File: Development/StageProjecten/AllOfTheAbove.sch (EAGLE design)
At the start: 90 parts, among them IC1 7809DT, IC2 TL074TSSOP14, IC3 TL074TSSOP14, IC4 TL074TSSOP14, IC5 UA741D, J1 JACK, J10 JACK, J11 JACK, J12 JACK, J13 JACK, J14 JACK, J15 JACK, J16 JACK, J2 POWERSHROUDED, J3 JACK, J4 JACK, J5 JACK, J6 JACK, J7 JACK, J8 JACK, J9 JACK

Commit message: Rat added with powerjumpers
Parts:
- added C29, C30, C31, C32, C33, C34, C35, C36, C37, C38, C39: (no value), OPL:C-0603
- added D13, D14: (no value), OPL:D-D1206
- added IC6: UA741D, linear:UA741D
- added JP1, JP2, JP3: (no value), pinhead:PINHD-1X3
- added Q1: SST201, transistor-fet:SST201
- added R22, R29, R30, R31: (no value), EurorackModularParts:POTSQUAREHOLE_SMALLKNOB
- added R32, R33, R34, R35, R36, R37, R38, R39, R40: (no value), OPL:R-0603
- D11, D12: device diode:DIODE-DO-214AC -> OPL:D-D1206
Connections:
- new net +4.5V: R34.2
- new net N$36: R22.E, R22.S, R28.1
- new net N$37: C29.2, JP1.2, R33.1
- new net N$38: C30.2, IC6.+IN, R33.2
- new net N$39: IC6.V+, JP2.2
- new net N$40: IC6.V-, JP3.2
- new net N$41: JP1.1, R34.1
- new net N$42: C31.1, IC6.-IN, R31.E, R31.S, R35.2, R36.2
- new net N$43: C31.2, C34.2, IC6.OUT, R31.A
- new net N$44: C34.1, R37.1
- new net N$45: D13.-, D14.+, R30.E, R30.S, R37.2
- new net N$46: R30.A, R38.1
- new net N$47: C33.2, R36.1
- new net N$48: C32.2, R35.1
- new net N$49: C35.1, C36.1, R38.2
- new net N$50: C36.2, Q1.G, R39.2
- new net N$51: C37.1, Q1.S, R40.2
- new net N$52: C37.2, R29.A
- net -12V: now also C39.1, JP3.3
- net 12V: now also C38.2, JP2.3
- net 9V: now also JP2.1, Q1.D
- net GND: now also C30.1, C32.1, C33.1, C35.2, C38.1, C39.2, D11.+, D12.-, D13.+, D14.-, JP3.1, R29.E, R32.2, R39.1, R40.1; no longer D11.A, D12.C
- net INPUT_B: now also C29.1, R32.1
- net N$21: now also IC5.+IN; no longer IC5.-IN
- net N$22: now also IC5.-IN; no longer IC5.+IN
- net N$34: now also D11.-, D12.+, R22.A; no longer D11.C, D12.A, R28.1

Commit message: Added FF&Muff schematic (.brd not updated)
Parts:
- added C40, C41, C42, C43, C44, C45, C46, C47, C48, C49, C50, C51, C52, C53, C54, C55: (no value), OPL:C-0603
- added D15, D16, D17, D18: (no value), OPL:D-D1206
- added Q2, Q3: BCX71SMD, transistor-pnp:BCX71SMD
- added Q4, Q5, Q6, Q7: BC849SMD, transistor-npn:BC849SMD
- added R41, R44, R45, R46, R47, R48, R49, R50, R51, R52, R53, R54, R55, R56, R57, R58, R59, R60, R61, R62, R63, R64, R65, R66, R67, R68: (no value), OPL:R-0603
- added R42, R43, R69, R70, R71: (no value), EurorackModularParts:POTSQUAREHOLE_SMALLKNOB
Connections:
- new net N$53: Q3.E, R41.1, R43.A
- new net N$54: C40.2, Q2.B, R41.2
- new net N$55: Q2.C, Q3.B, R45.2
- new net N$56: C41.1, R43.S
- new net N$57: C42.2, R42.A
- new net N$58: C42.1, R44.1, R46.2
- new net N$59: Q3.C, R44.2
- new net N$60: C43.1, R47.2
- new net N$61: C43.2, C44.1, Q4.B, R48.2, R49.2
- new net N$62: Q4.E, R50.1
- new net N$63: C44.2, C45.1, Q4.C, R49.1, R51.2
- new net N$64: C45.2, R71.A
- new net N$65: C47.1, C48.1, Q5.B, R53.2, R54.2, R56.2
- new net N$66: C48.2, D15.+, D16.-
- new net N$67: Q5.E, R55.2
- new net N$68: C47.2, C49.1, D15.-, D16.+, Q5.C, R56.1, R57.2
- new net N$69: C49.2, R58.1
- new net N$70: C50.1, C51.1, Q6.B, R58.2, R59.2, R61.2
- new net N$71: Q6.E, R60.2
- new net N$72: C50.2, C52.1, D17.-, D18.+, Q6.C, R61.1, R62.2, R63.1
- new net N$73: C53.1, R70.S
- new net N$74: C55.2, R63.2, R70.E
- new net N$75: C52.2, R64.1, R70.A
- new net N$76: C51.2, D17.+, D18.-
- new net N$77: C53.2, Q7.B, R65.2, R66.1
- new net N$78: C54.1, Q7.C, R67.1
- new net N$79: Q7.E, R68.2
- new net N$80: C54.2, R69.A
- new net N$84: R52.1, R71.E
- new net N$85: C46.2, R53.1
- new net N$86: C46.1, R71.S
- net 9V: now also R45.1, R46.1, R51.1, R57.1, R62.1, R66.2, R67.2
- net GND: now also C41.2, C55.1, Q2.E, R42.E, R43.E, R48.1, R50.2, R52.2, R54.1, R55.1, R59.1, R60.1, R64.2, R65.1, R68.1, R69.E
- net INPUT_C: now also C40.1
- net INPUT_D: now also R47.1
- net OUTPUT_B: now also R29.S
- net OUTPUT_C: now also R42.S
- net OUTPUT_D: now also R69.S

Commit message: Added Modules/Guitar In
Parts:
- removed C28, C29, C30, C31, C32, C33, C34, C35, C36, C37, C38, C39, C40, C41, C42, C43, C44, C45, C46, C47, C48, C49, C50, C51, C52, C53, C54, C55: (no value), OPL:C-0603
- removed D11, D12, D13, D14, D15, D16, D17, D18: (no value), OPL:D-D1206
- removed IC6: UA741D, linear:UA741D
- removed JP1, JP2, JP3: (no value), pinhead:PINHD-1X3
- removed Q1: SST201, transistor-fet:SST201
- removed Q2, Q3: BCX71SMD, transistor-pnp:BCX71SMD
- removed Q4, Q5, Q6, Q7: BC849SMD, transistor-npn:BC849SMD
- removed R27, R28, R32, R33, R34, R35, R36, R37, R38, R39, R40, R41, R44, R45, R46, R47, R48, R49, R50, R51, R52, R53, R54, R55, R56, R57, R58, R59, R60, R61, R62, R63, R64, R65, R66, R67, R68: (no value), OPL:R-0603
- removed R29, R30, R31, R42, R43, R69, R70, R71: (no value), EurorackModularParts:POTSQUAREHOLE_SMALLKNOB
- C22: value (none) -> 10uF
- IC5: value UA741D -> TL071D; device linear:UA741D -> EurorackModularParts:TL071D
- R22: value (none) -> 1M; device EurorackModularParts:POTSQUAREHOLE_SMALLKNOB -> OPL:R-0603; DESC Tone -> (none)
- R23: value 1M -> 150K; device EurorackModularParts:POTSQUAREHOLE_SMALLKNOB -> OPL:R-0603; DESC Distortion -> (none)
- R24: value 10K -> (none); device EurorackModularParts:POTSQUAREHOLE_SMALLKNOB -> OPL:R-0603; DESC Volume -> (none)
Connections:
- removed net +4.5V: R34.2
- removed net N$37: C29.2, JP1.2, R33.1
- removed net N$39: IC6.V+, JP2.2
- removed net N$40: IC6.V-, JP3.2
- removed net N$41: JP1.1, R34.1
- removed net N$42: C31.1, IC6.-IN, R31.E, R31.S, R35.2, R36.2
- removed net N$43: C31.2, C34.2, IC6.OUT, R31.A
- removed net N$44: C34.1, R37.1
- removed net N$45: D13.-, D14.+, R30.E, R30.S, R37.2
- removed net N$46: R30.A, R38.1
- removed net N$47: C33.2, R36.1
- removed net N$48: C32.2, R35.1
- removed net N$49: C35.1, C36.1, R38.2
- removed net N$50: C36.2, Q1.G, R39.2
- removed net N$51: C37.1, Q1.S, R40.2
- removed net N$52: C37.2, R29.A
- removed net N$53: Q3.E, R41.1, R43.A
- removed net N$54: C40.2, Q2.B, R41.2
- removed net N$55: Q2.C, Q3.B, R45.2
- removed net N$56: C41.1, R43.S
- removed net N$57: C42.2, R42.A
- removed net N$58: C42.1, R44.1, R46.2
- removed net N$59: Q3.C, R44.2
- removed net N$60: C43.1, R47.2
- removed net N$61: C43.2, C44.1, Q4.B, R48.2, R49.2
- removed net N$62: Q4.E, R50.1
- removed net N$63: C44.2, C45.1, Q4.C, R49.1, R51.2
- removed net N$64: C45.2, R71.A
- removed net N$65: C47.1, C48.1, Q5.B, R53.2, R54.2, R56.2
- removed net N$66: C48.2, D15.+, D16.-
- removed net N$67: Q5.E, R55.2
- removed net N$68: C47.2, C49.1, D15.-, D16.+, Q5.C, R56.1, R57.2
- removed net N$69: C49.2, R58.1
- removed net N$70: C50.1, C51.1, Q6.B, R58.2, R59.2, R61.2
- removed net N$71: Q6.E, R60.2
- removed net N$72: C50.2, C52.1, D17.-, D18.+, Q6.C, R61.1, R62.2, R63.1
- removed net N$73: C53.1, R70.S
- removed net N$74: C55.2, R63.2, R70.E
- removed net N$75: C52.2, R64.1, R70.A
- removed net N$76: C51.2, D17.+, D18.-
- removed net N$77: C53.2, Q7.B, R65.2, R66.1
- removed net N$78: C54.1, Q7.C, R67.1
- removed net N$79: Q7.E, R68.2
- removed net N$80: C54.2, R69.A
- removed net N$84: R52.1, R71.E
- removed net N$85: C46.2, R53.1
- removed net N$86: C46.1, R71.S
- new net BIASMAINLINE: C7.1, D2.ANODE, D4.ANODE, D6.ANODE, D7.ANODE, D8.ANODE, IC1.OUT, R13.1
- new net GUITAR_IN: C22.1, R22.2
- new net GUITAR_OUT: R26.2
- new net INPUT_E: R14.2
- new net N$81: IC5.V+
- new net N$82: IC5.V-
- new net OUTPUT_E: R22.1, R23.1
- net -12V: now also C27.1, C4.1, C6.1, IC1.V-, IC3SUPPLY.V-, R12.1, R9.2, U$13.-12V; no longer C39.1, IC5.V-, JP3.3
- net 12V: now also C26.2, C3.2, C5.2, IC1.V+, IC3SUPPLY.V+, R2.A; no longer C38.2, IC5.V+, JP2.3
- net 9V: no longer JP2.1, Q1.D, R45.1, R46.1, R51.1, R57.1, R62.1, R66.2, R67.2
- net GND: now also C23.1, C25.1, C26.1, C27.2, C3.1, C4.2, C6.2, D1.CATHODE, D10.CATHODE, D3.CATHODE, D5.CATHODE, D9.CATHODE, IC1.+IN, IC3BUF1.B, IC3BUF2.B, IC3OTA2.IN_N, IC3OTA2.IN_P, R1.E, R2.E, R22.1, R23.1, R24.2, R25.1, R26.1, R4.2, R5.2, R7.1, R8.1; no longer C28.1, C30.1, C32.1, C33.1, C35.2, C38.1, C39.2, C41.2, C55.1, D11.+, D12.-, D13.+, D14.-, JP3.1, Q2.E, R29.E, R32.2, R39.1, R40.1, R42.E, R43.E, R48.1, R50.2, R52.2, R54.1, R55.1, R59.1, R60.1, R64.2, R65.1, R68.1, R69.E
- net INPUT_B: no longer C29.1, R32.1
- net INPUT_C: no longer C40.1
- net INPUT_D: no longer R47.1
- net N$1: now also R4.1
- net N$10: now also R6.1
- net N$11: now also C8.1, IC1.OUT, R15.1, R16.2, R17.2
- net N$12: now also C14.2, C8.2, IC1.-IN, R15.2
- net N$13: now also C14.1, IC3OTA1.OUT, R5.1
- net N$14: now also D3.ANODE, D4.CATHODE, IC2A.+IN, R16.1
- net N$15: now also C9.1, IC2A.OUT, R18.1
- net N$16: now also D5.ANODE, D6.CATHODE, IC2B.+IN
- net N$17: now also C9.2, IC2A.-IN, R17.1, R18.2
- net N$18: now also C11.2, IC2C.-IN, R20.1
- net N$19: now also C16.1, IC1.OUT
- net N$20: now also C22.2, D8.CATHODE, D9.ANODE, IC2D.+IN, IC5.+IN, R23.2
- net N$21: now also C10.2, IC2B.-IN, R19.2
- net N$22: now also C10.1, C24.1, IC2B.OUT, IC5.OUT, R19.1, R20.2, R24.2, R26.1; no longer R27.1
- net N$23: now also C24.2, D10.ANODE, D7.CATHODE, IC2C.+IN, IC5.-IN, R24.1, R25.2
- net N$24: now also C11.1, IC2C.OUT
- net N$25: now also C13.1, IC1.+IN, R25.2
- net N$26: now also C15.2, IC2D.-IN, R21.2
- net N$27: now also C15.1, IC2D.OUT, R21.1
- net N$28: now also D1.ANODE, D2.CATHODE, IC1.+IN
- net N$29: now also C12.1, IC1.OUT, R22.2
- net N$3: now also C7.2, IC1.-IN, R13.2, R14.1
- net N$30: now also C16.2, IC1.-IN
- net N$32: now also C12.2, C25.2, IC1.-IN, R23.2, R24.1, R25.1; no longer R27.2
- net N$33: now also R9.1
- net N$34: now also IC3OTA1.I_BIAS, R6.2; no longer C28.2, D11.-, D12.+
- net N$35: no longer R28.2
- net N$36: now also IC3OTA1.IN_P, R7.2; no longer R28.1
- net N$38: now also IC3OTA1.IN_N, R8.2; no longer C30.2, IC6.+IN, R33.2
- net N$5: now also R1.S, R10.2
- net N$6: now also R1.A
- net N$7: now also R10.1, R11.1, R12.2
- net N$8: now also R11.2, R2.S
- net N$9: now also C13.2, R26.2
- net OUTPUT_B: no longer R29.S
- net OUTPUT_C: no longer R42.S
- net OUTPUT_D: no longer R69.S

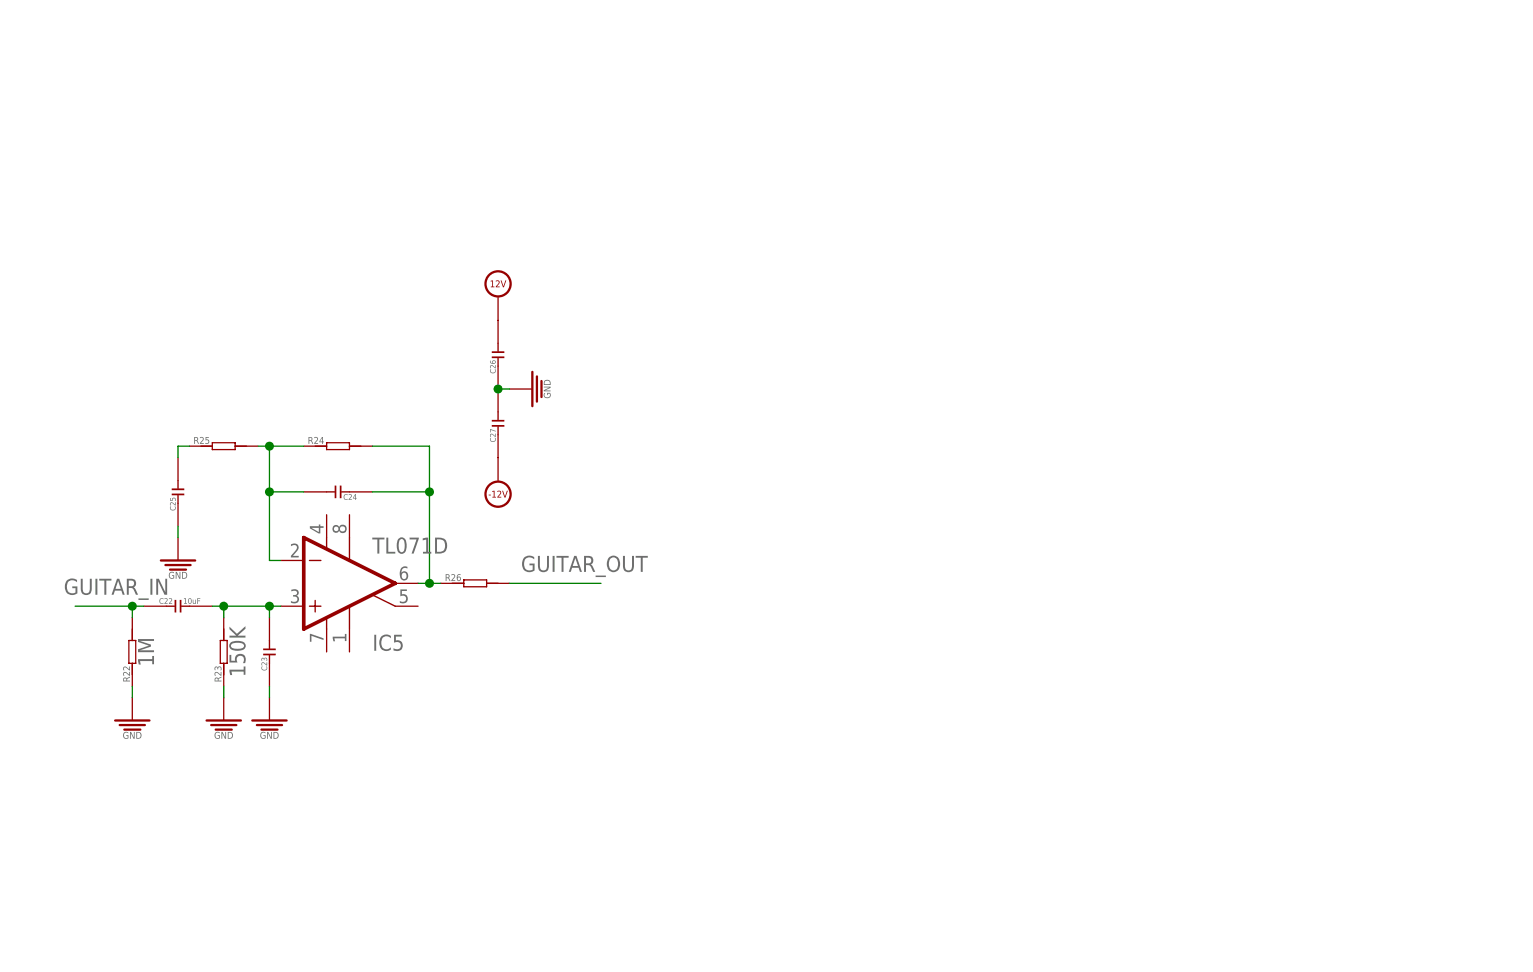
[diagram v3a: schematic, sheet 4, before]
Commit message: VCA added
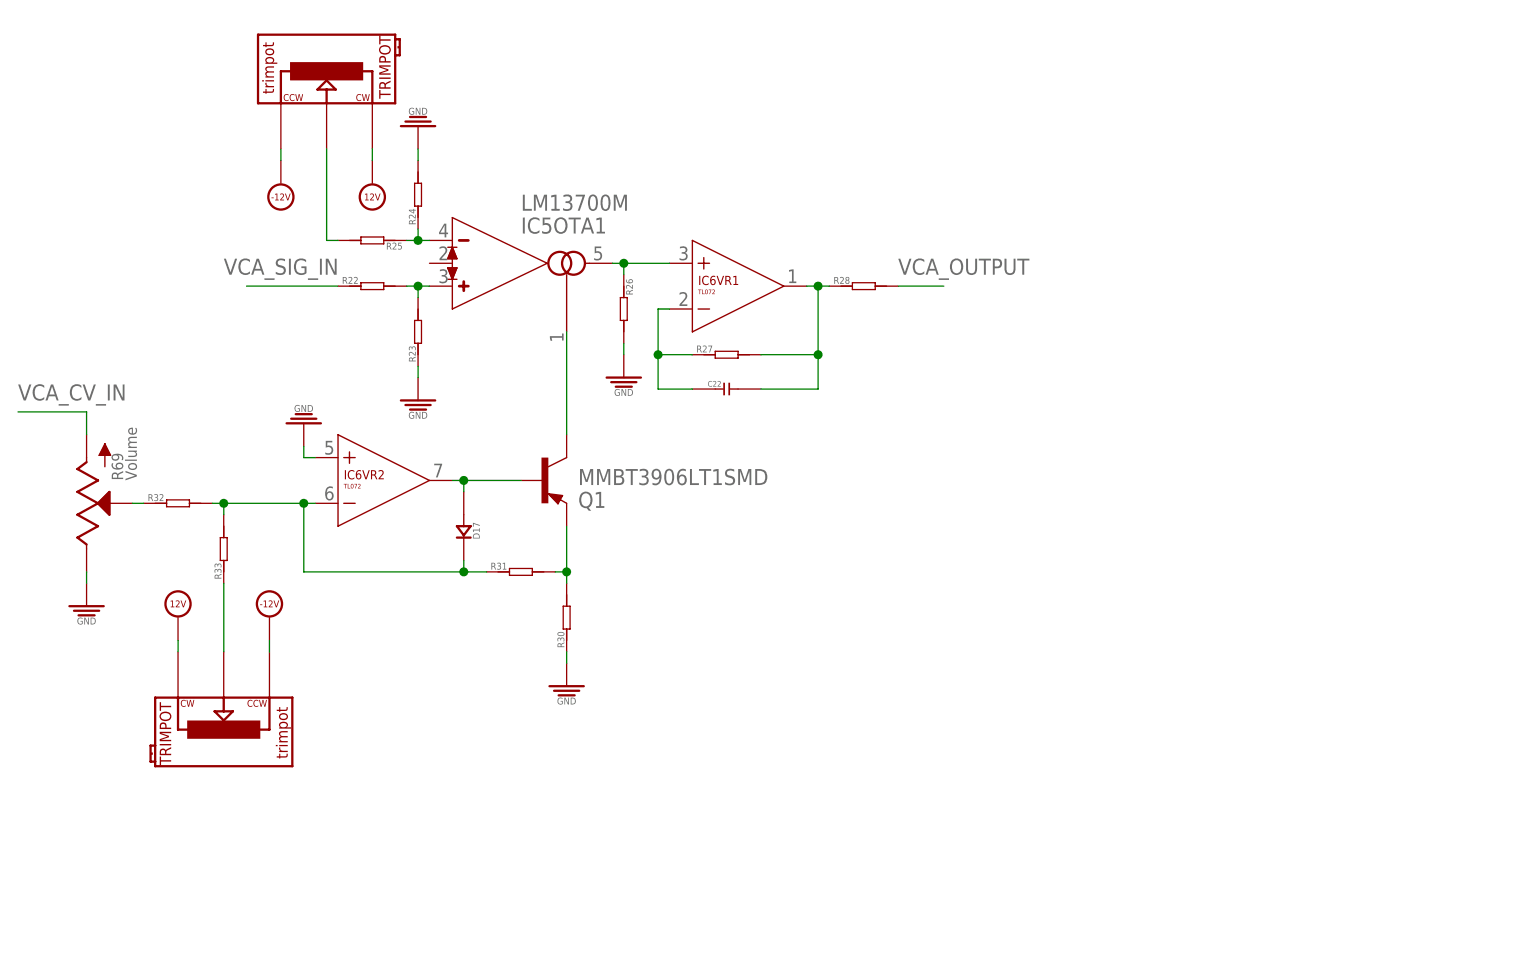
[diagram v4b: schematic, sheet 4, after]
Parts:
- removed C23, C24, C25, C26, C27: (no value), OPL:C-0603
- added D17: (no value), OPL:D-D1206
- added IC6: TL072, EurorackModularParts:TL072
- added Q1: MMBT3906LT1SMD, transistor-pnp:MMBT3906LT1SMD
- added R27, R28, R30, R31, R32, R33: (no value), OPL:R-0603
- added R29, R34: TRIMPOT, EurorackModularParts:TRIMPOT
- added R69: (no value), EurorackModularParts:POTSQUAREHOLE_SMALLKNOB
- C22: value 10uF -> (none)
- IC5: value TL071D -> LM13700M; device EurorackModularParts:TL071D -> ota:LM13700M
- R22: value 1M -> (none)
- R23: value 150K -> (none)
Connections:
- new net +4.5V: R34.2
- new net N$37: D17.-, IC6VR2.-IN, R31.1, R32.2, R33.1, R33.2
- new net N$39: IC5OTA1.I_BIAS, IC6A.V+, Q1.C
- new net N$40: IC6A.V-, R33.1, R34.P$2
- new net N$41: R34.1
- new net N$42: IC6A.-IN, R31.E, R31.S, R32.1, R69.S
- new net N$43: IC6A.OUT, R31.A
- new net N$45: R30.E, R30.S
- new net N$46: R30.A
- new net N$50: Q1.G
- new net N$51: Q1.S
- new net N$52: R29.A
- new net N$72: D17.-
- new net N$76: D17.+
- new net N$80: R69.A
- new net VCA_CV_IN: R69.A
- new net VCA_OUTPUT: R28.2
- new net VCA_SIG_IN: R22.1
- net -12V: now also IC5A.V-, R29.P$1, R34.P$1; no longer C25.1, C27.1
- net 12V: now also IC5A.V+, R29.P$3, R34.P$3; no longer C24.2, C26.2
- net 9V: now also Q1.D
- net GND: now also IC6VR2.+IN, R26.2, R29.E, R30.1, R32.2, R69.E; no longer C23.1, C24.1, C25.1, C25.2, C26.1, C27.2
- net GUITAR_IN: no longer C22.1
- net INPUT_A: no longer C23.1
- net INPUT_B: now also R32.1
- net N$15: now also R31.2, R32.2
- net N$16: now also R31.1
- net N$19: now also R27.1, R28.2
- net N$20: now also IC5A.+IN, IC5OTA1.IN_N, R24.1, R25.1, R34.1; no longer C22.2, C23.2, IC5.+IN
- net N$21: now also IC5A.+IN, IC5OTA1.IN_P, R22.2, R23.2, R32.1; no longer IC5.+IN
- net N$22: now also IC5A.-IN, IC5A.OUT, IC5OTA1.OUT, IC6VR1.+IN, R27.1, R33.2; no longer C24.1, C26.2, IC5.-IN, IC5.OUT
- net N$23: now also C22.1, IC5A.-IN, IC6VR1.-IN, R27.1, R33.1; no longer C24.2, C26.1, IC5.-IN
- net N$24: now also R34.2
- net N$27: now also R29.1, R30.1
- net N$28: now also R29.2
- net N$30: now also R28.1, R30.2
- net N$32: now also IC5A.OUT, R25.2, R27.2, R29.P$2; no longer C25.2, C27.1, IC5.OUT, R25.1
- net N$33: now also C22.2, IC6VR1.OUT, R27.2, R28.1
- net N$35: now also R28.2; no longer C27.2
- net N$36: now also D17.+, IC6VR2.OUT, Q1.B, R28.1
- net N$38: now also IC6A.+IN, Q1.E, R30.2, R31.2, R33.2
- net N$81: now also IC5A.V+; no longer IC5.V+
- net N$82: now also IC5A.V-; no longer IC5.V-
- net N$9: now also R27.2
- net OUTPUT_B: now also R29.S
- net OUTPUT_D: now also R69.S
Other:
- moved on the sheet: C22, R22, R23, R24, R25, R26
